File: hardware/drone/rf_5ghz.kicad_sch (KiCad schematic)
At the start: 18 parts, among them U7 CC3350, U8 DPX167125DT-8197B1, U9 DEA162450BT-1295A1, Y1 Crystal_GND24

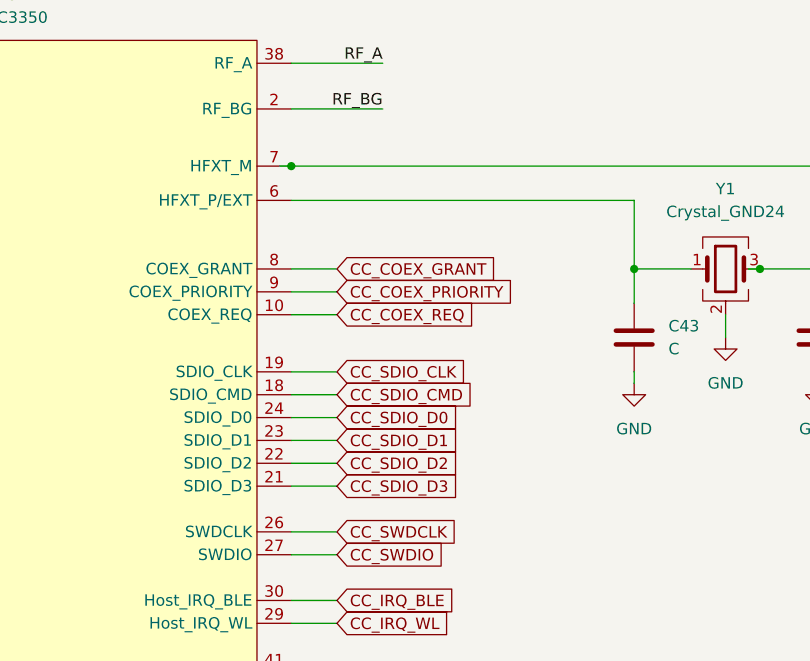
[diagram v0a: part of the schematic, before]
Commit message: more radio work
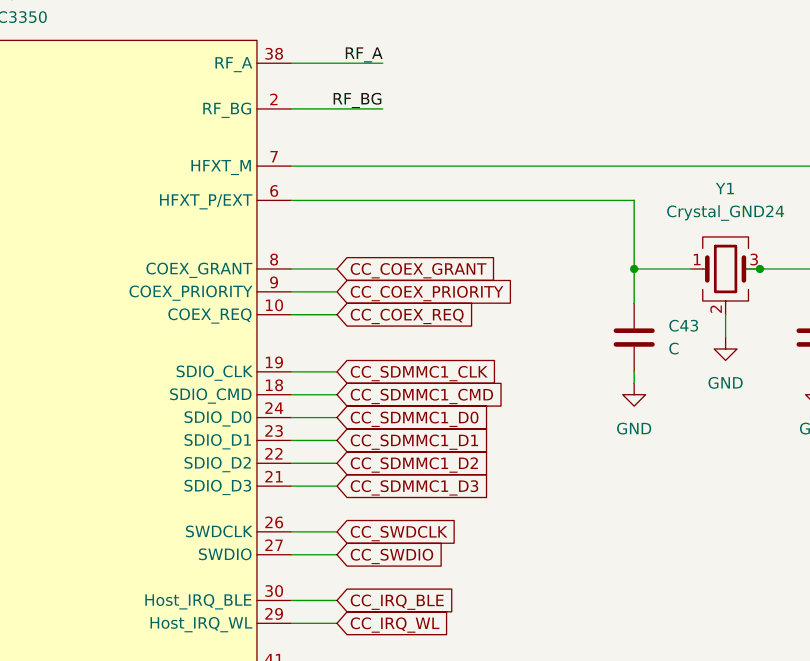
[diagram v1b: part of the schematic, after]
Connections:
- net CC_SDIO_CLK renamed CC_SDMMC1_CLK
- net CC_SDIO_CMD renamed CC_SDMMC1_CMD
- net CC_SDIO_D0 renamed CC_SDMMC1_D0
- net CC_SDIO_D1 renamed CC_SDMMC1_D1
- net CC_SDIO_D2 renamed CC_SDMMC1_D2
- net CC_SDIO_D3 renamed CC_SDMMC1_D3
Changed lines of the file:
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@@
-	)
-	(junction
-		(at 166.37 67.31)
-		(diameter 0)
-		(color 0 0 0 0)
 	)
 	(junction
@@
 	(wire
 		(pts
-			(xy 165.1 67.31) (xy 166.37 67.31)
-		)
-		(stroke
-			(width 0)
-			(type default)
-		)
-	)
-	(wire
-		(pts
 			(xy 55.88 77.47) (xy 55.88 78.74)
 		)
@@
 		)
 	)
-	(global_label "CC_SDIO_D1"
+	(global_label "CC_SDMMC1_D1"
 		(shape input)
 		(at 171.45 97.79 0)
@@
 		)
 		(property "Intersheetrefs" "${INTERSHEET_REFS}"
-			(at 185.8047 97.79 0)
+			(at 189.2517 97.79 0)
 			(hide yes)
 			(show_name no)
@@
 		)
 	)
-	(global_label "CC_SDIO_D3"
+	(global_label "CC_SDMMC1_D3"
 		(shape input)
 		(at 171.45 102.87 0)
@@
 		)
 		(property "Intersheetrefs" "${INTERSHEET_REFS}"
-			(at 185.8047 102.87 0)
+			(at 189.2517 102.87 0)
 			(hide yes)
 			(show_name no)
@@
 		)
 	)
-	(global_label "CC_SDIO_D0"
+	(global_label "CC_SDMMC1_D0"
 		(shape input)
 		(at 171.45 95.25 0)
@@
 		)
 		(property "Intersheetrefs" "${INTERSHEET_REFS}"
-			(at 185.8047 95.25 0)
+			(at 189.2517 95.25 0)
 			(hide yes)
 			(show_name no)
@@
 		)
 	)
-	(global_label "CC_SDIO_CMD"
+	(global_label "CC_SDMMC1_CMD"
 		(shape input)
 		(at 171.45 92.71 0)
@@
 		)
 		(property "Intersheetrefs" "${INTERSHEET_REFS}"
-			(at 187.3166 92.71 0)
+			(at 190.7636 92.71 0)
 			(hide yes)
 			(show_name no)
@@
 		)
 	)
-	(global_label "CC_SDIO_CLK"
+	(global_label "CC_SDMMC1_CLK"
 		(shape input)
 		(at 171.45 90.17 0)
@@
 		)
 		(property "Intersheetrefs" "${INTERSHEET_REFS}"
-			(at 186.8933 90.17 0)
+			(at 190.3403 90.17 0)
 			(hide yes)
 			(show_name no)
@@
 		)
 	)
-	(global_label "CC_SDIO_D2"
+	(global_label "CC_SDMMC1_D2"
 		(shape input)
 		(at 171.45 100.33 0)
@@
 		)
 		(property "Intersheetrefs" "${INTERSHEET_REFS}"
-			(at 185.8047 100.33 0)
-			(hide yes)
-			(show_name no)
+			(at 189.2517 100.33 0)
+			(hide yes)
+			(show_name no)
